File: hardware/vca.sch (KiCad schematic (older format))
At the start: 91 parts, among them P1 VCA_CMD_PWR, P10 CARD_2, P11 OUT_MAIN, P12 OUT_GND, P2 CARD_0, P3 CARD_1, P4 OUT_0, P5 OUT_1, P6 OUT_2, P7 OUT_3, P8 OUT_4, P9 OUT_5, U1 TL074, U10 TL082, U2 TL082, U3 4051, U4 SSM2164, U5 TL082, U6 TL082, U7 TL074, U8 SSM2164, U9 TL082

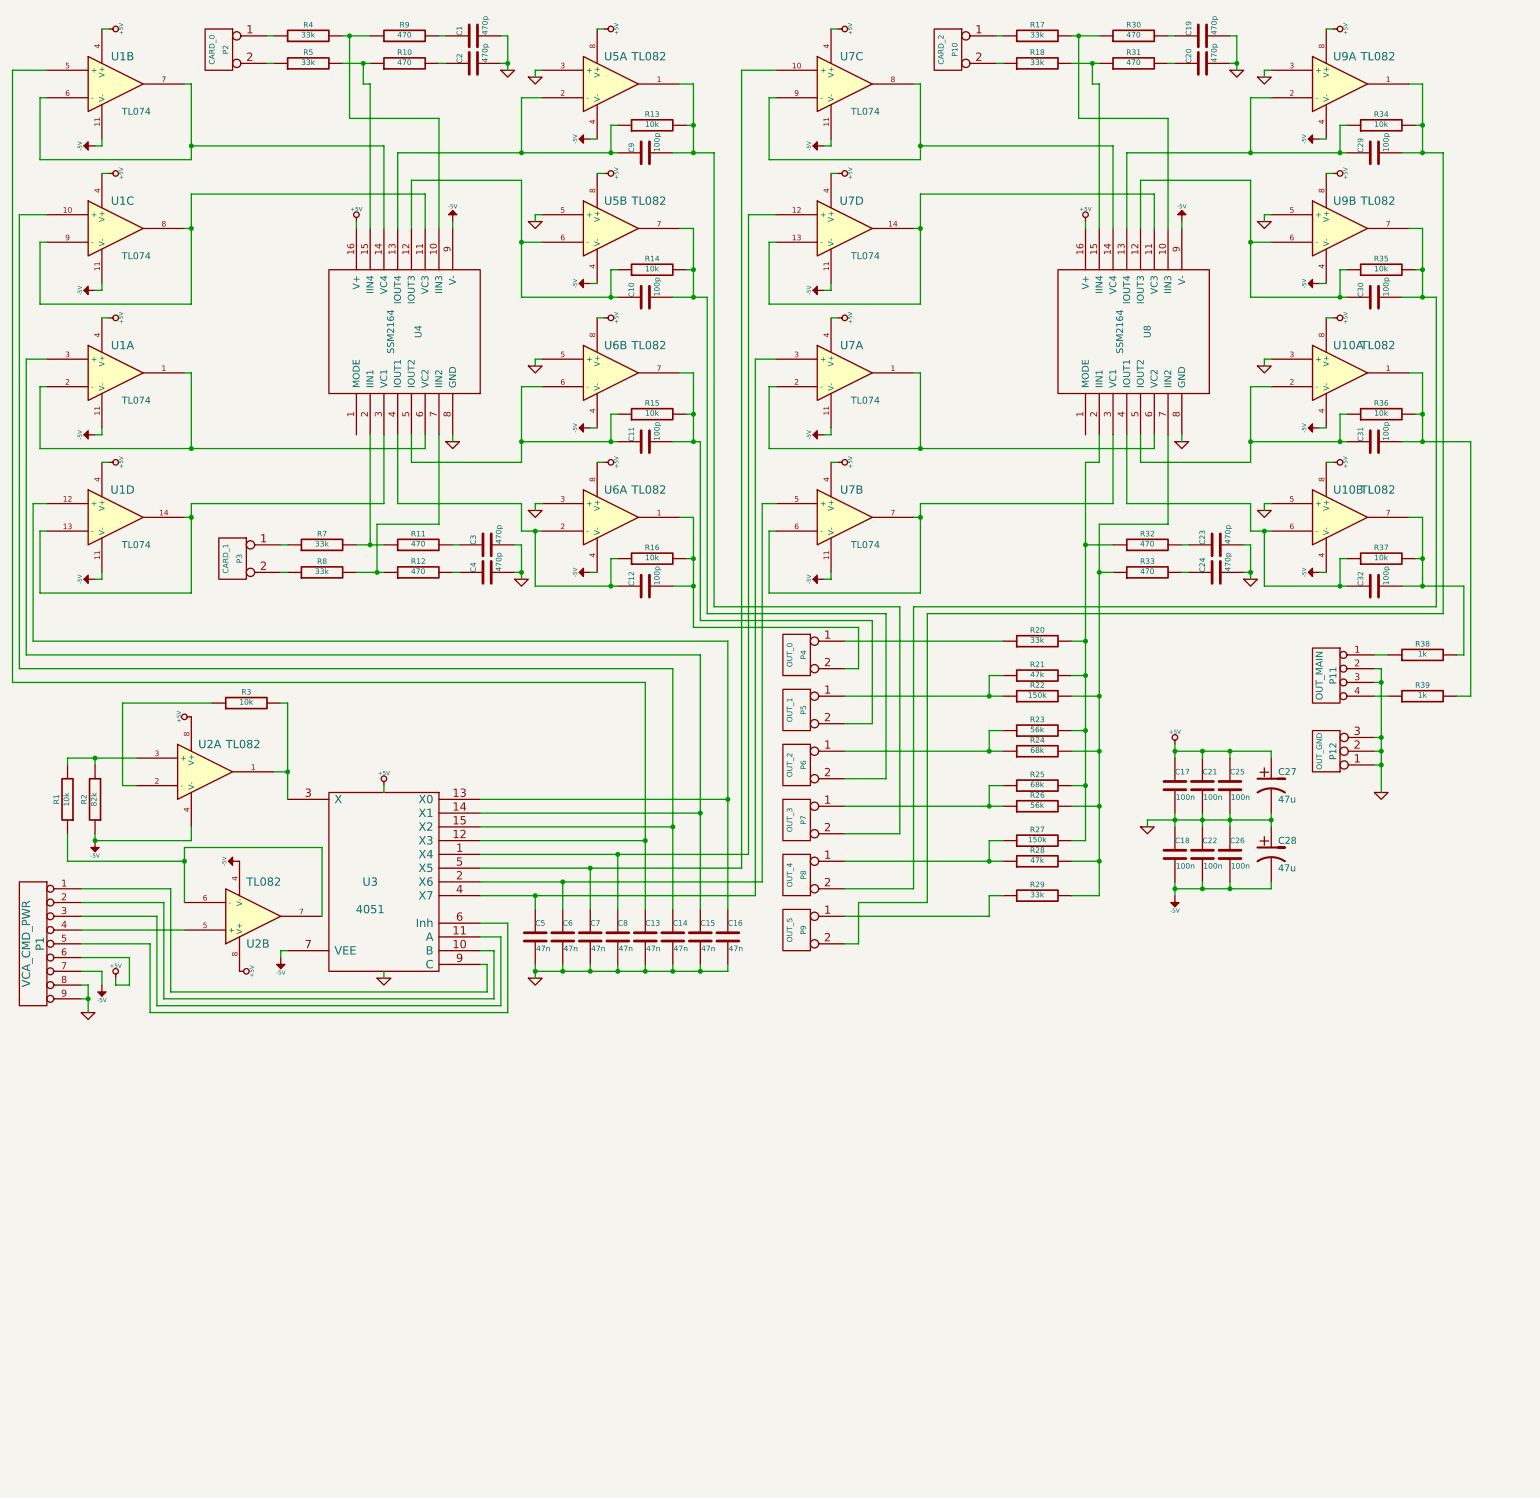
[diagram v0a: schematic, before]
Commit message: hw: new LM13700-based VCA / Mixer board schematics
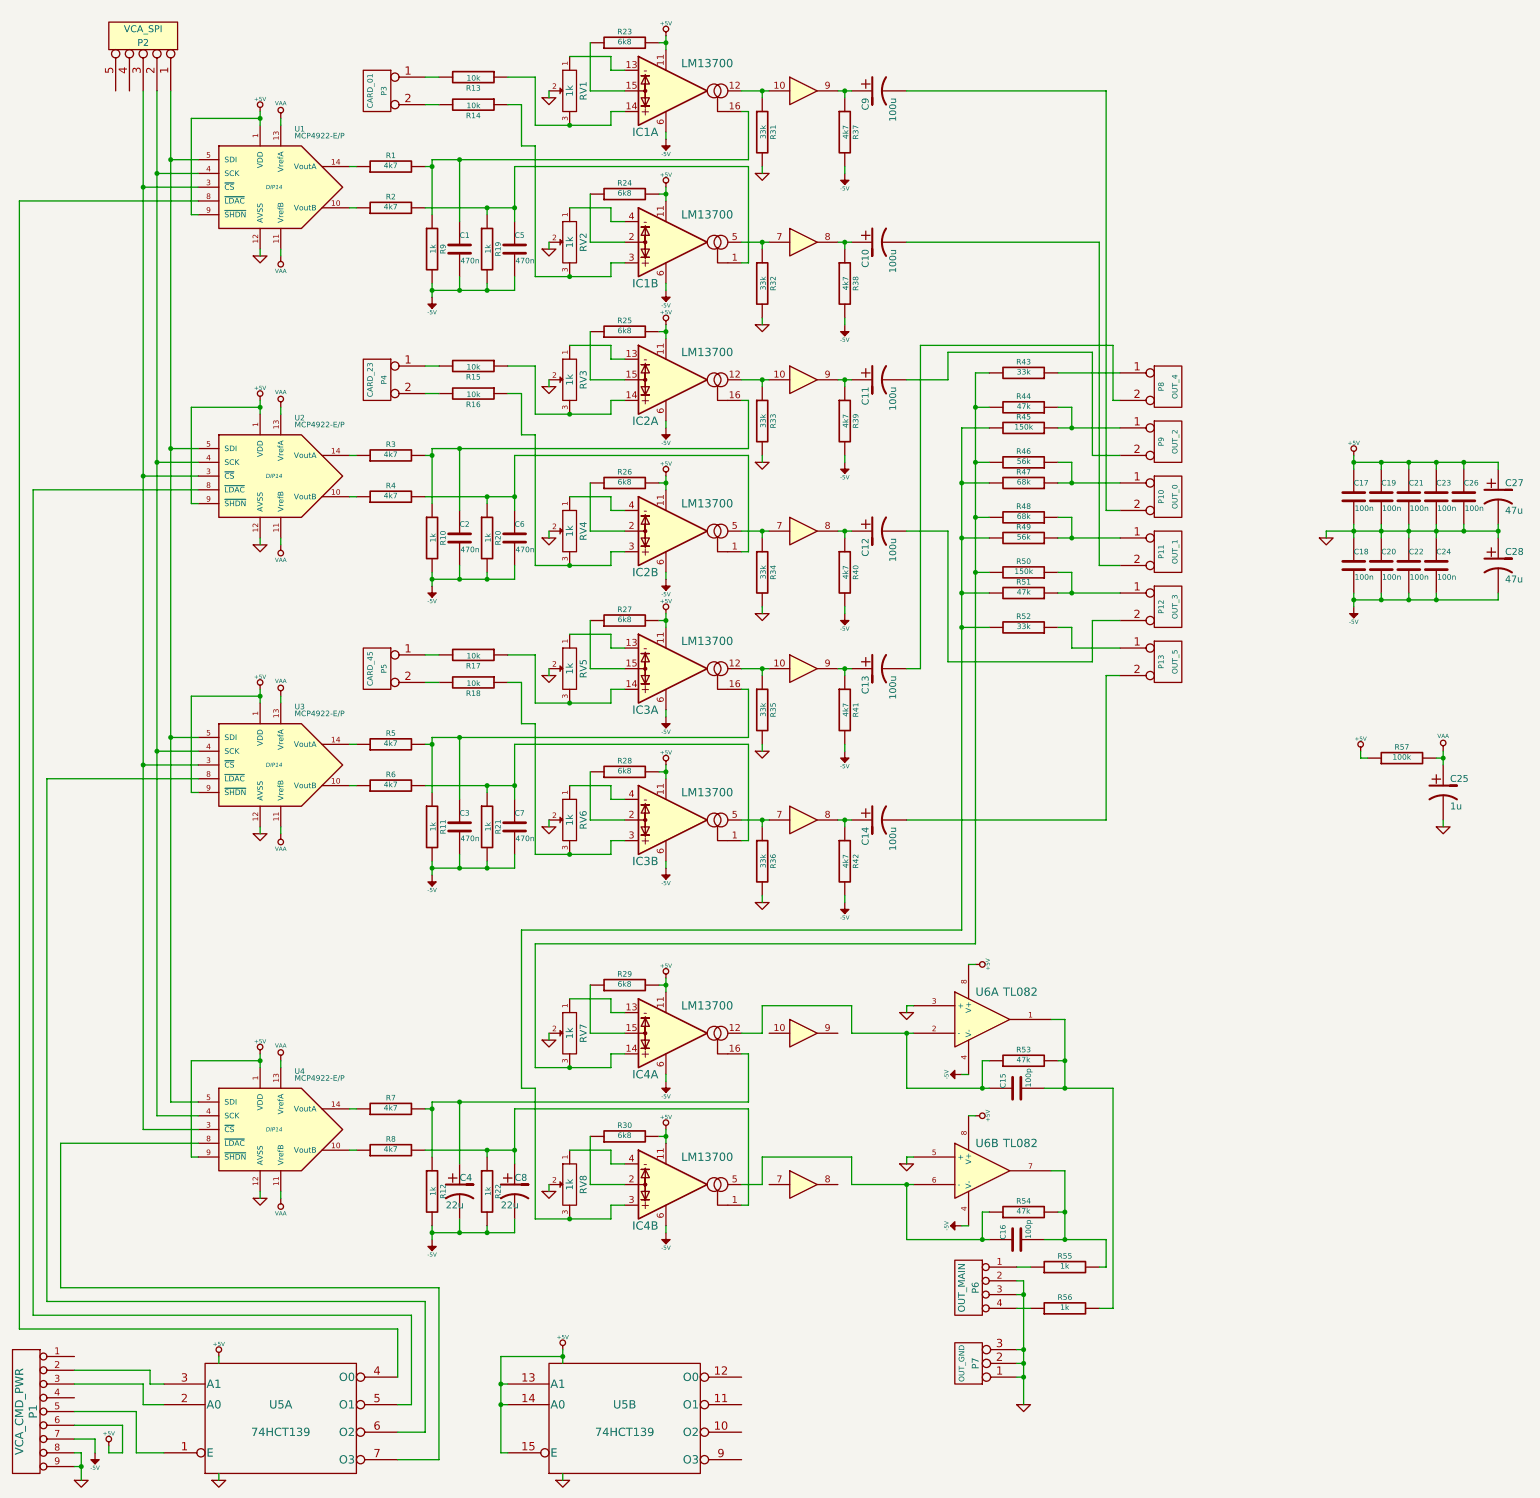
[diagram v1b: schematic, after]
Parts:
- removed C10, C11, C12, C29, C30, C9: 100p, ~, symbol C
- removed C13, C14, C15, C16, C8: 47n, ~, symbol C
- removed C19, C20, C4: 470p, ~, symbol C
- removed P10: CARD_2, symbol CONN_2
- removed P2: CARD_0, symbol CONN_2
- removed U1, U7: TL074, symbol TL074
- removed U2, U5, U6, U9: TL082, symbol TL082
- removed U3: 4051, symbol 4051
- removed U4, U8: SSM2164, MODULE, symbol SSM2164
- added C10, C11, C12, C13, C14, C9: 100u, ~, symbol CP1
- added C25: 1u, ~, symbol CP1
- added C26: 100n, ~, symbol C
- added C4, C8: 22u, ~, symbol CP1
- added IC1, IC2, IC3, IC4: LM13700, symbol LM13700
- added P2: VCA_SPI, symbol CONN_5
- added P4: CARD_23, symbol CONN_2
- added P5: CARD_45, symbol CONN_2
- added R19, R20, R21, R22: 1k, ~, symbol R
- added R23, R24, R25, R26, R27, R28, R29: 6k8, ~, symbol R
- added R36: 33k, ~, symbol R
- added R37, R38, R39, R40, R41, R42, R6: 4k7, ~, symbol R
- added R57: 100k, ~, symbol R
- added RV1, RV2, RV3, RV4, RV5, RV6, RV7, RV8: 1k, ~, symbol POT
- added U1, U2, U3, U4: MCP4922-E/P, DIP14, symbol MCP4922-E/P
- added U5: 74HCT139, ~, symbol 74LS139
- C1, C2, C3: value 470p -> 470n
- C23, C24: value 470p -> 100n
- C5, C6, C7: value 47n -> 470n
- P10: renamed from P6; value OUT_2 -> OUT_0
- P11: renamed from P7; value OUT_3 -> OUT_1
- P12: renamed from P8; value OUT_4 -> OUT_3
- P3: value CARD_1 -> CARD_01
- P8: renamed from P4; value OUT_0 -> OUT_4
- P9: renamed from P5; value OUT_1 -> OUT_2
- R1, R3: value 10k -> 4k7
- R10, R11, R12, R9: value 470 -> 1k
- R17, R18: value 33k -> 10k
- R2: value 82k -> 4k7
- R30: value 470 -> 6k8
- R31, R32, R33: value 470 -> 33k
- R34, R35: value 10k -> 33k
- R4, R5, R7, R8: value 33k -> 4k7
- R53: renamed from R36; value 10k -> 47k
- R54: renamed from R37; value 10k -> 47k
- renumbered C31 to C15, C32 to C16, C21 to C19, C22 to C20, C25 to C21, C26 to C22, P9 to P13, P11 to P6, P12 to P7, R20 to R43, R21 to R44, R22 to R45, R23 to R46, R24 to R47, R25 to R48, R26 to R49, R27 to R50, R28 to R51, R29 to R52, R38 to R55, R39 to R56, U10 to U6
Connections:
- net +5V: now also C23.1, R30.2, C26.1, IC1.11 (V+), IC1.11 (V+), IC2.11 (V+), IC2.11 (V+), IC3.11 (V+), IC3.11 (V+), IC4.11 (V+), IC4.11 (V+), R23.2, R24.2, R25.2, R26.2, R27.2, R28.2, R29.2, R57.1, U1.1 (VDD), U1.9 (~SHDN~), U2.1 (VDD), U2.9 (~SHDN~), U3.1 (VDD), U3.9 (~SHDN~), U4.1 (VDD), U4.9 (~SHDN~), U5.13 (A1), U5.14 (A0), U5.15 (E), U5.16 (VCC), U5.16 (VCC)
- net -5V: now also C1.2, C2.2, C24.2, C3.2, C5.2, C6.2, C7.2, R10.2, R11.2, R12.2, R9.2, C4.2, C8.2, IC1.6 (V-), IC1.6 (V-), IC2.6 (V-), IC2.6 (V-), IC3.6 (V-), IC3.6 (V-), IC4.6 (V-), IC4.6 (V-), R19.2, R20.2, R21.2, R22.2, R37.2, R38.2, R39.2, R40.2, R41.2, R42.2; no longer R2.1
- net GND: now also C24.1, R31.2, R32.2, R33.2, R34.2, R35.2, C25.2, C26.2, R36.2, RV1.2, RV2.2, RV3.2, RV4.2, RV5.2, RV6.2, RV7.2, RV8.2, U1.12 (AVSS), U2.12 (AVSS), U3.12 (AVSS), U4.12 (AVSS), U5.8 (GND), U5.8 (GND); no longer C1.2, C2.2, C24.2, C3.2, C5.2, C6.2, C7.2
- net at P1.2 (P2): now also U5.3 (A1)
- net at P1.3 (P3): now also U5.2 (A0)
- net at C6.1: now also R4.2, IC2.1 (Iabc), R20.1
- net at R3.2: now also C2.1, R10.1, IC2.16 (Iabc)
- net at C5.1: now also R2.2, IC1.1 (Iabc), R19.1
- net at C7.1: now also IC3.1 (Iabc), R21.1, R6.2
- net at P1.5 (P5): now also U5.1 (E)
- net at R9.1: now also C1.1, R1.2, IC1.16 (Iabc); no longer R4.2
- net at R14.1: now also IC1.3 (+), RV2.3
- net at R13.1: now also IC1.14 (+), RV1.3
- net at R5.2: now also C3.1, R11.1, IC3.16 (Iabc); no longer R10.1
- net at R7.2: now also R12.1, C4.1, IC4.16 (Iabc); no longer R11.1
- net at R16.1: now also IC2.3 (+), RV4.3
- net at R15.1: now also IC2.14 (+), RV3.3
- net at R8.2: now also C8.1, IC4.1 (Iabc), R22.1; no longer R12.1
- net at P11.2 (PM): now also C10.2; no longer R13.2
- net at P3.1 (P1): now also R13.2; no longer R7.1
- net at P3.2 (PM): now also R14.2; no longer R8.1
- net at P10.2 (PM): now also C9.2; no longer R14.2
- net at P9.2 (PM): now also C11.2; no longer R15.2
- net at P8.2 (PM): now also C13.2; no longer R16.2
- net at R4.1: now also U2.10 (VoutB)
- net at R5.1: now also U3.14 (VoutA)
- net at R45.2, R47.2, R49.2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: now also IC4.3 (+), RV8.3; no longer R33.1
- net at R43.2, R44.2, R46.2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: now also IC4.14 (+), RV7.3; no longer R32.1
- net at R1.1: now also U1.14 (VoutA)
- net at R3.1: now also U2.14 (VoutA)
- net at R17.2: now also P5.1 (P1); no longer R30.1
- net at R35.1: now also IC3.10 (buffer_in), IC3.12 (out)
- net at R34.1: now also IC2.5 (out), IC2.7 (buffer_in)
- net at R31.1: now also IC1.10 (buffer_in), IC1.12 (out); no longer R18.2
- net at C16.1, R54.1, U6.6 (-): now also IC4.5 (out)
- net at C15.1, R53.1, U6.2 (-): now also IC4.12 (out)
- net at P13.2 (PM): now also C14.2; no longer R34.2
- net at P12.2 (PM): now also C12.2; no longer R35.2
- net at R17.1: now also IC3.14 (+), RV5.3
- net at R18.1: now also IC3.3 (+), RV6.3
- new net: P2.1, U1.5 (SDI), U2.5 (SDI), U3.5 (SDI), U4.5 (SDI)
- new net: P2.2, U1.4 (SCK), U2.4 (SCK), U3.4 (SCK), U4.4 (SCK)
- new net: P2.3, U1.3 (~CS~), U2.3 (~CS~), U3.3 (~CS~), U4.3 (~CS~)
- new net: R2.1, U1.10 (VoutB)
- new net: U1.8 (~LDAC~), U5.4 (O0)
- new net: IC1.13 (-), RV1.1
- new net: IC1.15 (bias), R23.1
- new net: C9.1, IC1.9 (buffer_out), R37.1
- new net: U2.8 (~LDAC~), U5.5 (O1)
- new net: U3.8 (~LDAC~), U5.6 (O2)
- new net: U4.8 (~LDAC~), U5.7 (O3)
- new net: IC1.2 (bias), R24.1
- new net: IC1.4 (-), RV2.1
- new net: IC1.5 (out), IC1.7 (buffer_in), R32.1
- new net: C10.1, IC1.8 (buffer_out), R38.1
- new net: IC2.10 (buffer_in), IC2.12 (out), R33.1
- new net: IC2.13 (-), RV3.1
- new net: IC2.15 (bias), R25.1
- new net: C11.1, IC2.9 (buffer_out), R39.1
- new net: IC2.2 (bias), R26.1
- new net: IC2.4 (-), RV4.1
- new net: C12.1, IC2.8 (buffer_out), R40.1
- new net: P4.1 (P1), R15.2
- new net: P4.2 (PM), R16.2
- new net: R6.1, U3.10 (VoutB)
- new net: IC3.13 (-), RV5.1
- new net: IC3.15 (bias), R27.1
- new net: C13.1, IC3.9 (buffer_out), R41.1
- new net: IC3.2 (bias), R28.1
- new net: IC3.4 (-), RV6.1
- new net: IC3.5 (out), IC3.7 (buffer_in), R36.1
- new net: C14.1, IC3.8 (buffer_out), R42.1
- new net: P5.2 (PM), R18.2
- new net: R8.1, U4.10 (VoutB)
- new net: R7.1, U4.14 (VoutA)
- new net: IC4.13 (-), RV7.1
- new net: IC4.15 (bias), R29.1
- new net: IC4.2 (bias), R30.1
- new net: IC4.4 (-), RV8.1
- new net VAA: C25.1, R57.2, U1.11 (VrefB), U1.13 (VrefA), U2.11 (VrefB), U2.13 (VrefA), U3.11 (VrefB), U3.13 (VrefA), U4.11 (VrefB), U4.13 (VrefA)
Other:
- moved on the sheet: C15, C16, C17, C18, C19, C20, C21, C22, C27, C28, P1, P10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
